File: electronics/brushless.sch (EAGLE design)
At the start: 63 parts, among them J1 USB_MINI-B_SMT, X1 JST-XH-10-PIN-LONG-PAD

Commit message: mos (wip)
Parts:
- added Q1, Q2, Q3, Q4, Q5, Q6: BUK7Y12-40E, transistor-power:BUK7Y12-40E
- R1, R10, R11, R12, R14, R15, R16, R17, R18, R19, R2, R20, R21, R22, R23, R24, R25, R3, R4, R5, R6, R7, R8, R9: device rhoban:RESISTANCE-R0805 -> SparkFun-Resistors:RESISTOR0805
- R28, R29, R35, R36, R39, R40, R48, R49, R50: device SparkFun-Passives:RESISTOR0805-RES -> SparkFun-Resistors:RESISTOR0805
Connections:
- net GND: now also Q2.S, Q4.S, Q6.S
- net N$1: now also Q1.G
- net N$2: now also Q3.G
- net N$3: now also Q2.G
- net N$6: now also Q4.G
- net N$7: now also Q5.G
- net N$9: now also Q6.G
- net U_PHASE: now also Q1.S, Q2.D
- net V+: now also Q1.D, Q3.D, Q5.D
- net V_PHASE: now also Q3.S, Q4.D
- net W_PHASE: now also Q5.S, Q6.D

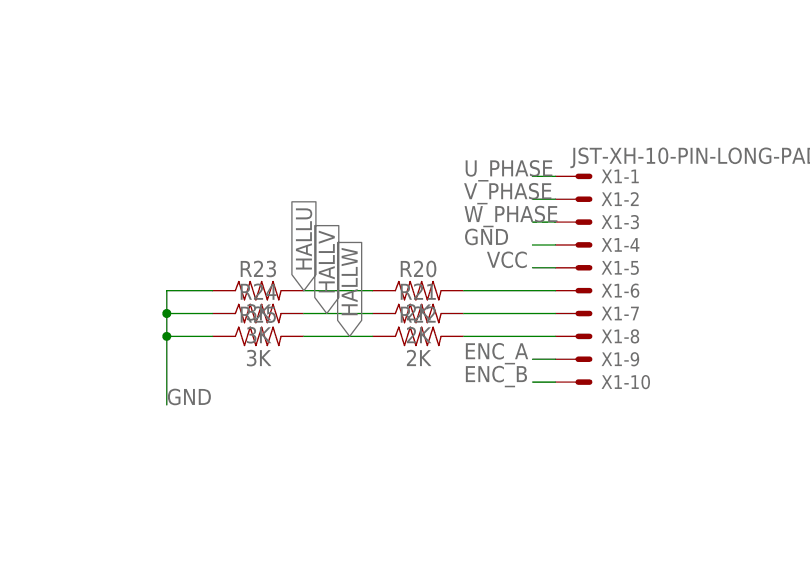
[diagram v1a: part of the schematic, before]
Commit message: tweak
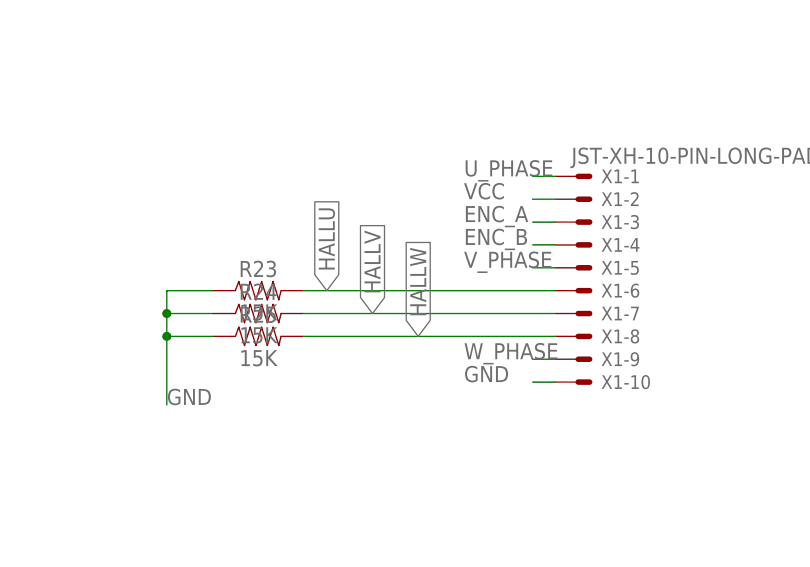
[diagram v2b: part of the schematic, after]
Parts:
- removed R20, R21, R22: 2K, SparkFun-Resistors:RESISTOR0805
- R23, R24, R25: value 3K -> 15K
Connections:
- removed net HALL1: R20.2, X1-6.S
- removed net HALL2: R21.2, X1-7.S
- removed net HALL3: R22.2, X1-8.S
- net ENC_A: now also X1-3.S; no longer X1-9.S
- net ENC_B: now also X1-4.S; no longer X1-10.S
- net GND: now also X1-10.S; no longer X1-4.S
- net HALLU: now also X1-6.S; no longer R20.1
- net HALLV: now also X1-7.S; no longer R21.1
- net HALLW: now also X1-8.S; no longer R22.1
- net VCC: now also X1-2.S; no longer X1-5.S
- net V_PHASE: now also X1-5.S; no longer X1-2.S
- net W_PHASE: now also X1-9.S; no longer X1-3.S
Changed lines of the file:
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@@
 <class number="0" name="default" width="0" drill="0">
 </class>
-<class number="2" name="power" width="0.762" drill="0">
+<class number="2" name="power" width="0" drill="0">
 </class>
 </classes>
@@
 <part name="U$5" library="rhoban" deviceset="CONNEC_1X08" device=""/>
 <part name="X1" library="Rembrandt Electronics - JST XH Connectors v1-0" deviceset="JST-XH-10-PIN" device="-LONG-PAD"/>
-<part name="R20" library="SparkFun-Resistors" deviceset="RESISTOR" device="0805" value="2K"/>
-<part name="R21" library="SparkFun-Resistors" deviceset="RESISTOR" device="0805" value="2K"/>
-<part name="R22" library="SparkFun-Resistors" deviceset="RESISTOR" device="0805" value="2K"/>
-<part name="R23" library="SparkFun-Resistors" deviceset="RESISTOR" device="0805" value="3K"/>
-<part name="R24" library="SparkFun-Resistors" deviceset="RESISTOR" device="0805" value="3K"/>
-<part name="R25" library="SparkFun-Resistors" deviceset="RESISTOR" device="0805" value="3K"/>
+<part name="R23" library="SparkFun-Resistors" deviceset="RESISTOR" device="0805" value="15K"/>
+<part name="R24" library="SparkFun-Resistors" deviceset="RESISTOR" device="0805" value="15K"/>
+<part name="R25" library="SparkFun-Resistors" deviceset="RESISTOR" device="0805" value="15K"/>
 <part name="Q1" library="transistor-power" deviceset="BUK7Y12-40E" device=""/>
 <part name="Q3" library="transistor-power" deviceset="BUK7Y12-40E" device=""/>
@@
 <instance part="X1" gate="-9" x="144.78" y="-66.04"/>
 <instance part="X1" gate="-10" x="144.78" y="-68.58"/>
-<instance part="R20" gate="G$1" x="127" y="-58.42"/>
-<instance part="R21" gate="G$1" x="127" y="-60.96"/>
-<instance part="R22" gate="G$1" x="127" y="-63.5"/>
 <instance part="R23" gate="G$1" x="109.22" y="-58.42"/>
 <instance part="R24" gate="G$1" x="109.22" y="-60.96"/>
@@
 </segment>
 <segment>
-<pinref part="X1" gate="-4" pin="S"/>
-<wire x1="142.24" y1="-53.34" x2="139.7" y2="-53.34" width="0.1524" layer="91"/>
-<label x="132.08" y="-53.34" size="1.778" layer="95"/>
-</segment>
-<segment>
 <pinref part="R23" gate="G$1" pin="1"/>
 <wire x1="104.14" y1="-58.42" x2="99.06" y2="-58.42" width="0.1524" layer="91"/>
@@
 <label x="99.06" y="-71.12" size="1.778" layer="95"/>
 </segment>
+<segment>
+<pinref part="X1" gate="-10" pin="S"/>
+<wire x1="142.24" y1="-68.58" x2="139.7" y2="-68.58" width="0.1524" layer="91"/>
+<label x="132.08" y="-68.58" size="1.778" layer="95"/>
+</segment>
 </net>
 <net name="U_GATE_HIGH" class="0">
@@
 </segment>
 <segment>
-<pinref part="X1" gate="-2" pin="S"/>
-<wire x1="142.24" y1="-48.26" x2="139.7" y2="-48.26" width="0.1524" layer="91"/>
-<label x="132.08" y="-48.26" size="1.778" layer="95"/>
+<pinref part="X1" gate="-5" pin="S"/>
+<wire x1="142.24" y1="-55.88" x2="139.7" y2="-55.88" width="0.1524" layer="91"/>
+<label x="132.08" y="-55.88" size="1.778" layer="95"/>
 </segment>
 </net>
@@
 </segment>
 <segment>
-<pinref part="X1" gate="-3" pin="S"/>
-<wire x1="142.24" y1="-50.8" x2="139.7" y2="-50.8" width="0.1524" layer="91"/>
-<label x="132.08" y="-50.8" size="1.778" layer="95"/>
+<pinref part="X1" gate="-9" pin="S"/>
+<wire x1="142.24" y1="-66.04" x2="139.7" y2="-66.04" width="0.1524" layer="91"/>
+<label x="132.08" y="-66.04" size="1.778" layer="95"/>
 </segment>
 </net>
@@
 </segment>
 <segment>
-<pinref part="X1" gate="-5" pin="S"/>
-<wire x1="142.24" y1="-55.88" x2="139.7" y2="-55.88" width="0.1524" layer="91"/>
-<label x="134.62" y="-55.88" size="1.778" layer="95"/>
-</segment>
-<segment>
 <pinref part="U$4" gate="G$1" pin="IN"/>
 <wire x1="-302.26" y1="86.36" x2="-304.8" y2="86.36" width="0.1524" layer="91"/>
 <label x="-304.8" y="86.36" size="1.778" layer="95" rot="R180" xref="yes"/>
+</segment>
+<segment>
+<pinref part="X1" gate="-2" pin="S"/>
+<wire x1="142.24" y1="-48.26" x2="139.7" y2="-48.26" width="0.1524" layer="91"/>
+<label x="132.08" y="-48.26" size="1.778" layer="95"/>
 </segment>
 </net>
@@
 <net name="ENC_A" class="0">
 <segment>
-<pinref part="X1" gate="-9" pin="S"/>
-<wire x1="142.24" y1="-66.04" x2="139.7" y2="-66.04" width="0.1524" layer="91"/>
-<label x="132.08" y="-66.04" size="1.778" layer="95"/>
-</segment>
-<segment>
 <pinref part="ENC1" gate="G$1" pin="A"/>
 <wire x1="-165.1" y1="-66.04" x2="-162.56" y2="-66.04" width="0.1524" layer="91"/>
 <label x="-162.56" y="-66.04" size="1.778" layer="95"/>
 </segment>
-</net>
-<net name="HALL3" class="0">
-<segment>
-<pinref part="X1" gate="-8" pin="S"/>
-<wire x1="142.24" y1="-63.5" x2="132.08" y2="-63.5" width="0.1524" layer="91"/>
-<pinref part="R22" gate="G$1" pin="2"/>
-</segment>
-</net>
-<net name="HALL2" class="0">
-<segment>
-<pinref part="X1" gate="-7" pin="S"/>
-<wire x1="142.24" y1="-60.96" x2="132.08" y2="-60.96" width="0.1524" layer="91"/>
-<pinref part="R21" gate="G$1" pin="2"/>
-</segment>
-</net>
-<net name="HALL1" class="0">
-<segment>
+<segment>
+<pinref part="X1" gate="-3" pin="S"/>
+<wire x1="142.24" y1="-50.8" x2="139.7" y2="-50.8" width="0.1524" layer="91"/>
+<label x="132.08" y="-50.8" size="1.778" layer="95"/>
+</segment>
+</net>
+<net name="HALLU" class="0">
+<segment>
+<pinref part="R23" gate="G$1" pin="2"/>
 <pinref part="X1" gate="-6" pin="S"/>
-<wire x1="142.24" y1="-58.42" x2="132.08" y2="-58.42" width="0.1524" layer="91"/>
-<pinref part="R20" gate="G$1" pin="2"/>
-</segment>
-</net>
-<net name="HALLU" class="0">
-<segment>
-<pinref part="R20" gate="G$1" pin="1"/>
-<pinref part="R23" gate="G$1" pin="2"/>
-<wire x1="114.3" y1="-58.42" x2="121.92" y2="-58.42" width="0.1524" layer="91"/>
-<label x="114.3" y="-58.42" size="1.778" layer="95" rot="R90" xref="yes"/>
+<wire x1="114.3" y1="-58.42" x2="142.24" y2="-58.42" width="0.1524" layer="91"/>
+<label x="116.84" y="-58.42" size="1.778" layer="95" rot="R90" xref="yes"/>
 </segment>
 <segment>
@@
 <net name="HALLV" class="0">
 <segment>
-<pinref part="R21" gate="G$1" pin="1"/>
-<pinref part="R24" gate="G$1" pin="2"/>
-<wire x1="114.3" y1="-60.96" x2="121.92" y2="-60.96" width="0.1524" layer="91"/>
-<label x="116.84" y="-60.96" size="1.778" layer="95" rot="R90" xref="yes"/>
-</segment>
-<segment>
 <pinref part="UC1" gate="G$1" pin="PA5/SPI1_SCK/ADC12_IN5"/>
 <wire x1="-185.42" y1="22.86" x2="-187.96" y2="22.86" width="0.1524" layer="91"/>
 <label x="-187.96" y="22.86" size="1.27" layer="95" rot="R180" xref="yes"/>
 </segment>
+<segment>
+<pinref part="X1" gate="-7" pin="S"/>
+<pinref part="R24" gate="G$1" pin="2"/>
+<label x="121.92" y="-60.96" size="1.778" layer="95" rot="R90" xref="yes"/>
+<wire x1="142.24" y1="-60.96" x2="114.3" y2="-60.96" width="0.1524" layer="91"/>
+</segment>
 </net>
 <net name="HALLW" class="0">
-<segment>
-<pinref part="R22" gate="G$1" pin="1"/>
-<pinref part="R25" gate="G$1" pin="2"/>
-<wire x1="114.3" y1="-63.5" x2="121.92" y2="-63.5" width="0.1524" layer="91"/>
-<label x="119.38" y="-63.5" size="1.778" layer="95" rot="R90" xref="yes"/>
-</segment>
 <segment>
 <pinref part="UC1" gate="G$1" pin="PA6/SPI1_MISO/ADC12_IN6/TIM3_CH1"/>
@@
 <label x="-187.96" y="20.32" size="1.27" layer="95" rot="R180" xref="yes"/>
 </segment>
+<segment>
+<pinref part="X1" gate="-8" pin="S"/>
+<pinref part="R25" gate="G$1" pin="2"/>
+<label x="127" y="-63.5" size="1.778" layer="95" rot="R90" xref="yes"/>
+<wire x1="142.24" y1="-63.5" x2="114.3" y2="-63.5" width="0.1524" layer="91"/>
+</segment>
 </net>
 <net name="ENC_B" class="0">
@@
 </segment>
 <segment>
-<pinref part="X1" gate="-10" pin="S"/>
-<wire x1="142.24" y1="-68.58" x2="139.7" y2="-68.58" width="0.1524" layer="91"/>
-<label x="132.08" y="-68.58" size="1.778" layer="95"/>
-</segment>
-</net>
+<pinref part="X1" gate="-4" pin="S"/>
+<wire x1="142.24" y1="-53.34" x2="139.7" y2="-53.34" width="0.1524" layer="91"/>
+<label x="132.08" y="-53.34" size="1.778" layer="95"/>
+</segment>
+</net>

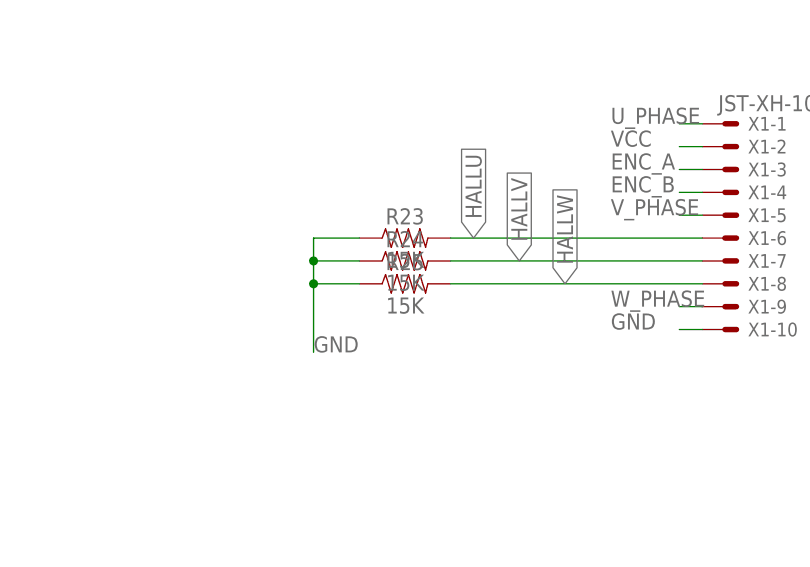
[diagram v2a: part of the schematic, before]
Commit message: up
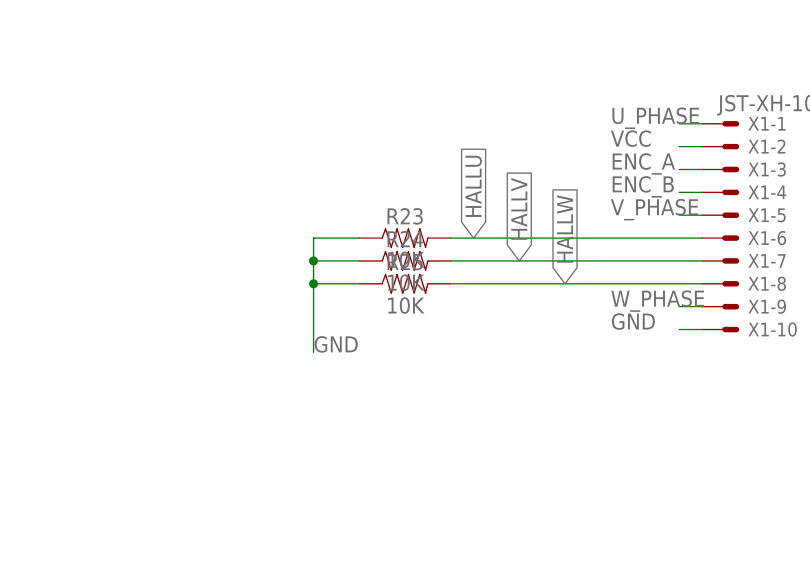
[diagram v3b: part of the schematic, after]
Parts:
- R23, R24, R25: value 15K -> 10K
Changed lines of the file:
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@@
 <part name="U$5" library="rhoban" deviceset="CONNEC_1X08" device=""/>
 <part name="X1" library="Rembrandt Electronics - JST XH Connectors v1-0" deviceset="JST-XH-10-PIN" device="-LONG-PAD"/>
-<part name="R23" library="SparkFun-Resistors" deviceset="RESISTOR" device="0805" value="15K"/>
-<part name="R24" library="SparkFun-Resistors" deviceset="RESISTOR" device="0805" value="15K"/>
-<part name="R25" library="SparkFun-Resistors" deviceset="RESISTOR" device="0805" value="15K"/>
+<part name="R23" library="SparkFun-Resistors" deviceset="RESISTOR" device="0805" value="10K"/>
+<part name="R24" library="SparkFun-Resistors" deviceset="RESISTOR" device="0805" value="10K"/>
+<part name="R25" library="SparkFun-Resistors" deviceset="RESISTOR" device="0805" value="10K"/>
 <part name="Q1" library="transistor-power" deviceset="BUK7Y12-40E" device=""/>
 <part name="Q3" library="transistor-power" deviceset="BUK7Y12-40E" device=""/>

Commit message: wip
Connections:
- net RX1: now also UC1.PA10/USART1_RX/TIM1_CH3
- net TX1: now also UC1.PA9/USART1_TX/TIM1_CH2
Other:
- note added: "CONNECTORS"
- note added: "MCU"
- note removed: "STM32"

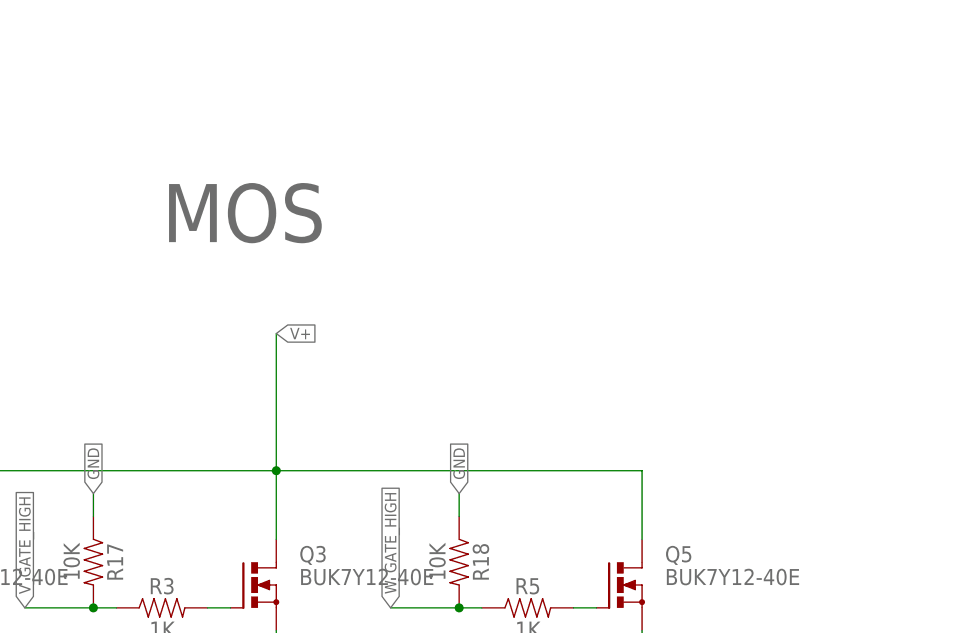
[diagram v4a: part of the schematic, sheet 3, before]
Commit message: bl wip
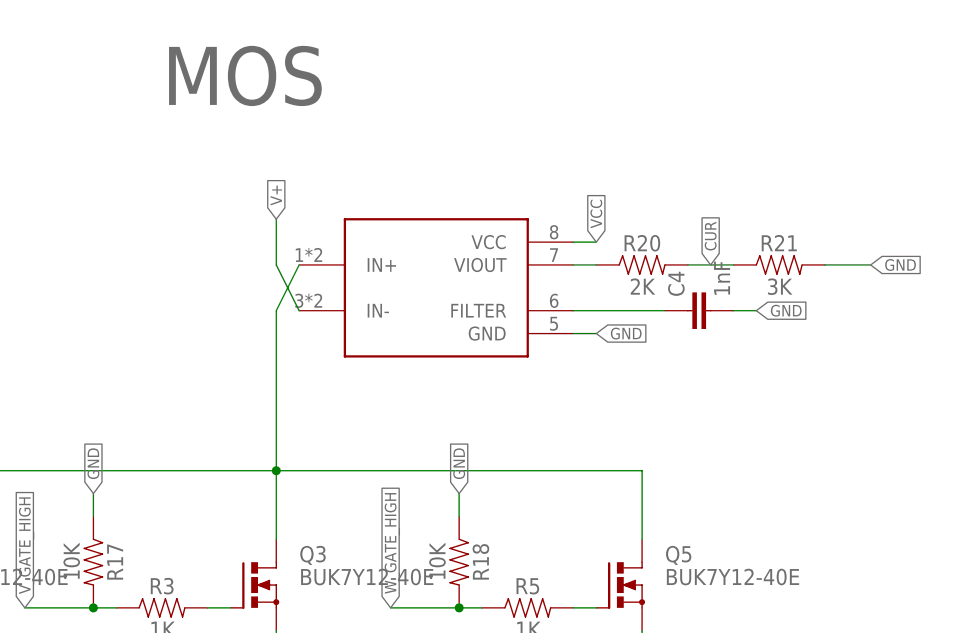
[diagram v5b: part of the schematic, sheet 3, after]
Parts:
- removed PROGRAM: CONNEC_1X066PADS, rhoban:CONNEC_1X066PADS
- removed XTAL1: 40Mhz, rhoban:QUARTZ
- added C4: 1nF, SparkFun-Passives:CAP0805
- added OSC1: 40Mhz, SparkFun2:CRYSTAL5X3
- added R20: 2K, SparkFun-Resistors:RESISTOR0805
- added R21: 3K, SparkFun-Resistors:RESISTOR0805
- added U$7: ACS712, rhoban:ACS712
- D1, D2, D3: FARNELL (none) -> 2317446
- U$1, U$2, U$3: FARNELL (none) -> 2296000
- UC1: FARNELL (none) -> 1606327
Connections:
- new net CUR: R20.2, R21.1, UC1.PA7/SPI1_MOSI/ADC12_IN7/TIM3_CH2
- new net N$24: R20.1, U$7.VIOUT
- new net N$27: C4.1, U$7.FILTER
- new net V+_MOS: Q1.D, Q3.D, Q5.D, U$7.IN+
- net 3.3: no longer PROGRAM.2
- net BOOT1: no longer PROGRAM.4
- net GND: now also C4.2, R21.2, U$7.GND; no longer PROGRAM.1
- net N$20: now also OSC1.1; no longer XTAL1.2
- net N$21: now also OSC1.2; no longer XTAL1.1
- net RESET: no longer PROGRAM.3
- net RX1: no longer PROGRAM.6
- net TX1: no longer PROGRAM.5
- net V+: now also U$7.IN-; no longer Q1.D, Q3.D, Q5.D
- net VCC: now also U$7.VCC

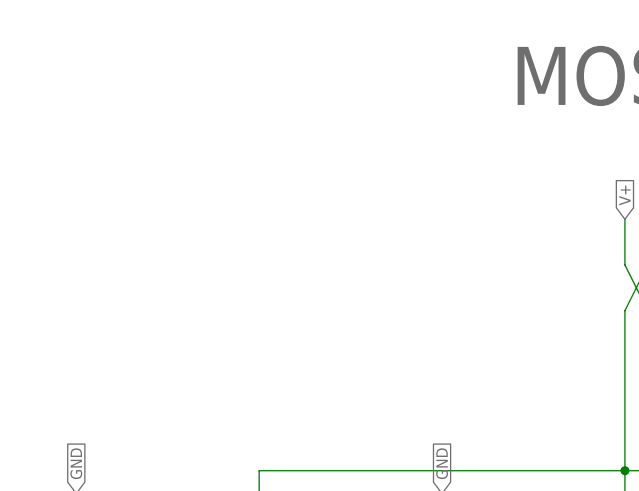
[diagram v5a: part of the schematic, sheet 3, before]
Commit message: Controller board
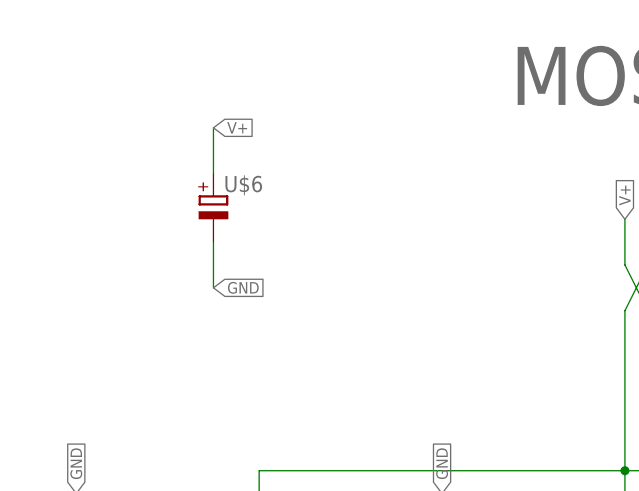
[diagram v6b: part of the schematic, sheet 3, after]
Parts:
- added U$6: (no value), rhoban:CPOL_EU_3.5-8
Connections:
- net ENC_B: now also X1-5.S; no longer X1-4.S
- net GND: now also U$6.-
- net HALLV: now also X1-9.S; no longer X1-7.S
- net V+: now also U$6.+
- net V_PHASE: now also X1-4.S; no longer X1-5.S
- net W_PHASE: now also X1-7.S; no longer X1-9.S
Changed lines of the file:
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@@
 <attribute name="VALUE" value=" "/>
 </part>
+<part name="U$6" library="rhoban" deviceset="CPOL_EU" device="_3.5-8"/>
 </parts>
 <sheets>
@@
 <instance part="R20" gate="G$1" x="111.76" y="83.82"/>
 <instance part="R21" gate="G$1" x="127" y="83.82"/>
+<instance part="U$6" gate="G$1" x="25.4" y="88.9"/>
 </instances>
 <busses>
@@
 <label x="137.16" y="83.82" size="1.27" layer="95" xref="yes"/>
 </segment>
+<segment>
+<pinref part="U$6" gate="G$1" pin="-"/>
+<wire x1="25.4" y1="86.36" x2="25.4" y2="81.28" width="0.1524" layer="91"/>
+<label x="25.4" y="81.28" size="1.27" layer="95" xref="yes"/>
+</segment>
 </net>
 <net name="U_GATE_HIGH" class="0">
@@
 <pinref part="U$7" gate="G$1" pin="IN-"/>
 <wire x1="73.66" y1="78.74" x2="71.12" y2="83.82" width="0.1524" layer="91"/>
+</segment>
+<segment>
+<pinref part="U$6" gate="G$1" pin="+"/>
+<wire x1="25.4" y1="93.98" x2="25.4" y2="99.06" width="0.1524" layer="91"/>
+<label x="25.4" y="99.06" size="1.27" layer="95" xref="yes"/>
 </segment>
 </net>
@@
 </segment>
 </net>
-<net name="V_PHASE" class="2">
-<segment>
-<pinref part="X1" gate="-5" pin="S"/>
-<wire x1="10.16" y1="-5.08" x2="7.62" y2="-5.08" width="0.1524" layer="91"/>
-<label x="7.62" y="-5.08" size="1.27" layer="95" rot="R180" xref="yes"/>
-</segment>
-</net>
 <net name="W_PHASE" class="2">
 <segment>
-<pinref part="X1" gate="-9" pin="S"/>
-<wire x1="10.16" y1="-15.24" x2="7.62" y2="-15.24" width="0.1524" layer="91"/>
-<label x="7.62" y="-15.24" size="1.27" layer="95" rot="R180" xref="yes"/>
+<pinref part="X1" gate="-7" pin="S"/>
+<wire x1="10.16" y1="-10.16" x2="7.62" y2="-10.16" width="0.1524" layer="91"/>
+<label x="7.62" y="-10.16" size="1.27" layer="95" rot="R180" xref="yes"/>
 </segment>
 </net>
@@
 </segment>
 </net>
-<net name="HALLV" class="0">
-<segment>
-<pinref part="X1" gate="-7" pin="S"/>
-<pinref part="R24" gate="G$1" pin="2"/>
-<label x="-15.24" y="-10.16" size="1.27" layer="95" rot="R90" xref="yes"/>
-<wire x1="10.16" y1="-10.16" x2="-17.78" y2="-10.16" width="0.1524" layer="91"/>
-</segment>
-</net>
 <net name="HALLW" class="0">
 <segment>
@@
 <net name="ENC_B" class="0">
 <segment>
-<pinref part="X1" gate="-4" pin="S"/>
-<wire x1="10.16" y1="-2.54" x2="7.62" y2="-2.54" width="0.1524" layer="91"/>
-<label x="7.62" y="-2.54" size="1.27" layer="95" rot="R180" xref="yes"/>
+<pinref part="X1" gate="-5" pin="S"/>
+<wire x1="10.16" y1="-5.08" x2="7.62" y2="-5.08" width="0.1524" layer="91"/>
+<label x="7.62" y="-5.08" size="1.27" layer="95" rot="R180" xref="yes"/>
 </segment>
 </net>
@@
 </segment>
 </net>
+<net name="HALLV" class="0">
+<segment>
+<pinref part="X1" gate="-9" pin="S"/>
+<wire x1="10.16" y1="-15.24" x2="-10.16" y2="-15.24" width="0.1524" layer="91"/>
+<wire x1="-10.16" y1="-15.24" x2="-10.16" y2="-10.16" width="0.1524" layer="91"/>
+<pinref part="R24" gate="G$1" pin="2"/>
+<wire x1="-10.16" y1="-10.16" x2="-17.78" y2="-10.16" width="0.1524" layer="91"/>
+<label x="-15.24" y="-10.16" size="1.27" layer="95" rot="R90" xref="yes"/>
+</segment>
+</net>
+<net name="V_PHASE" class="2">
+<segment>
+<pinref part="X1" gate="-4" pin="S"/>
+<wire x1="10.16" y1="-2.54" x2="7.62" y2="-2.54" width="0.1524" layer="91"/>
+<label x="7.62" y="-2.54" size="1.27" layer="95" rot="R180" xref="yes"/>
+</segment>
+</net>
